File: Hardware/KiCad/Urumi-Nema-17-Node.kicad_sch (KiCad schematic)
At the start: 64 parts, among them J1 B3B-XH-A, J3 Input, J4 B4B-XH-A_LF__SN_, J5 B4B-XH-A_LF__SN_, J6 Output, J8 PinHeader_01x05_P2.54mm_Horiz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, M0 SolderJumper_2_Open, M1 SolderJumper_2_Open, M2 SolderJumper_2_Open, Q2 SS8050, SW1 Switch_Tactile_CnK, U1 Microcontroller_AVR128DB32-I_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, U3 DRV8825_STEPPER_MOTOR_DRIVER_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, U5 MAX485E, Y1 16_MHz_Crystal

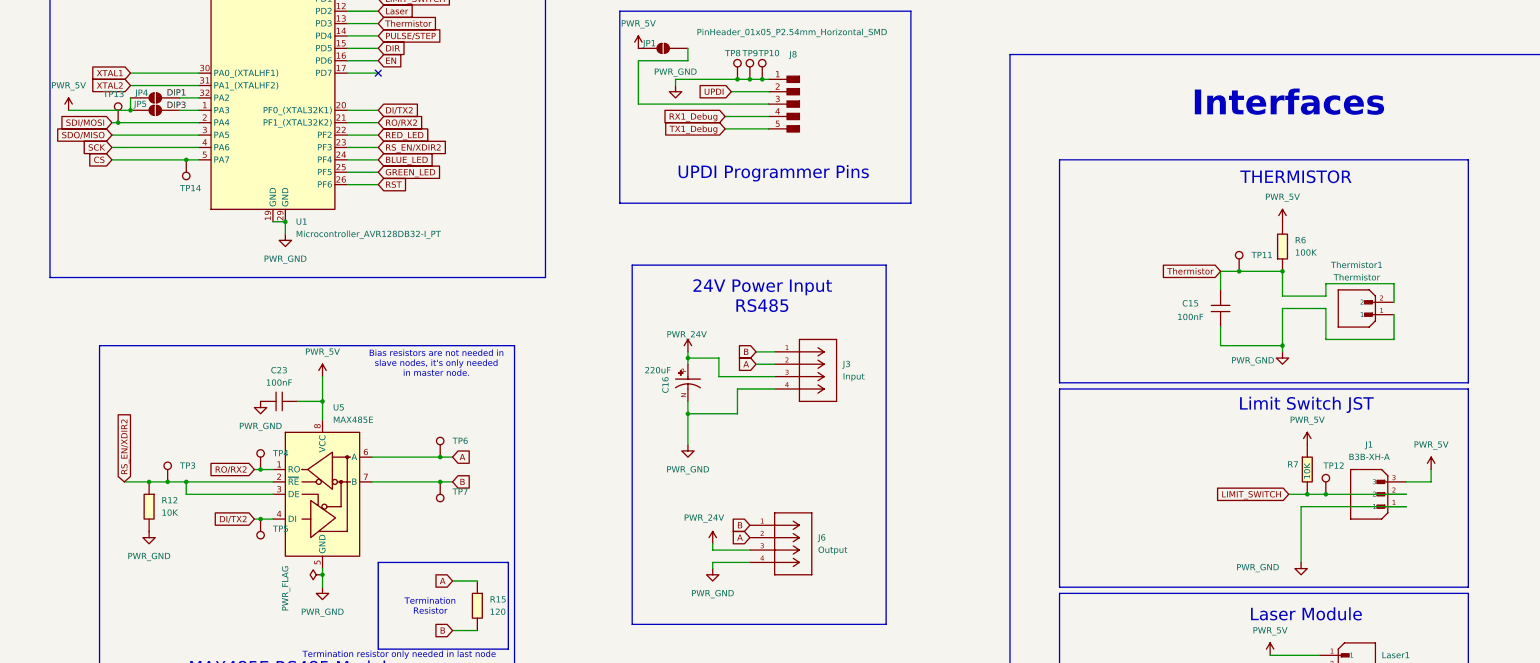
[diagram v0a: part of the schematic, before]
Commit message: hw: final V1.1.0
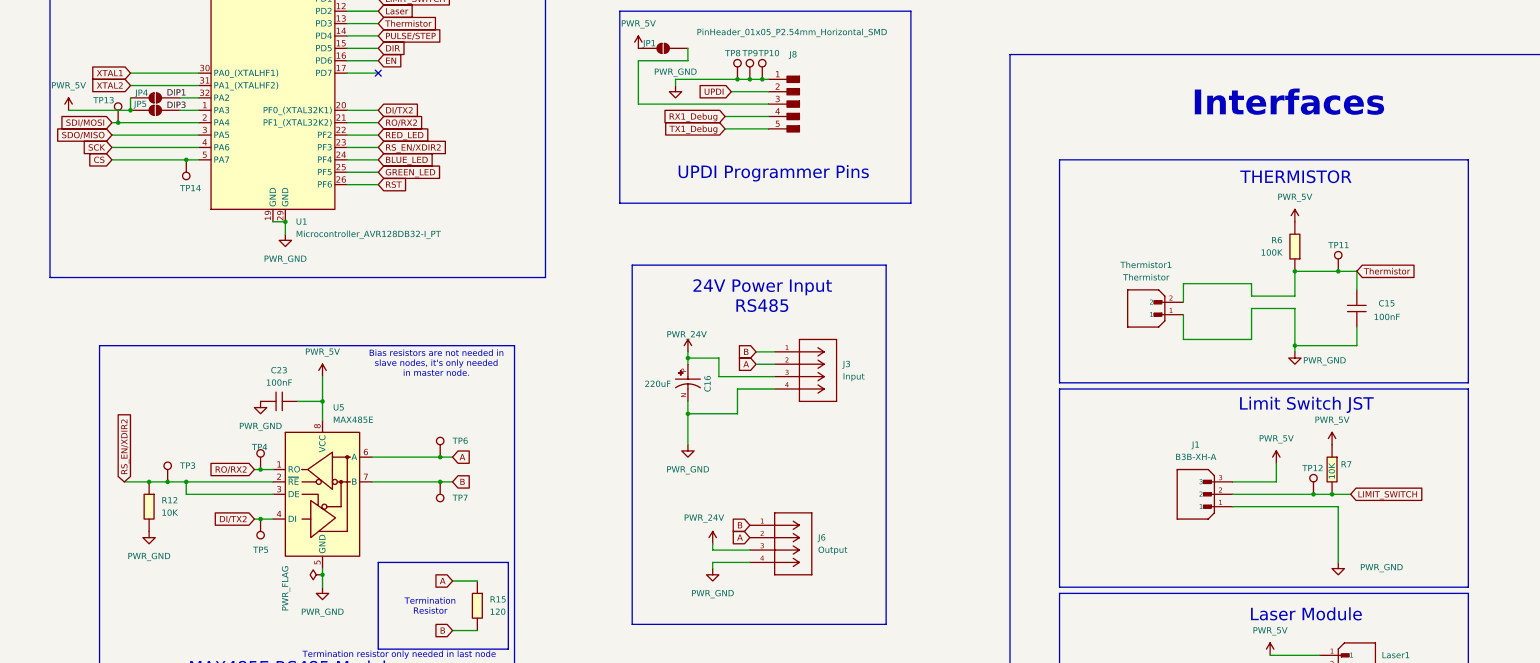
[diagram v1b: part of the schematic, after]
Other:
- moved on the sheet: C15, J1, R6, R7, TP11, TP12, Thermistor1
